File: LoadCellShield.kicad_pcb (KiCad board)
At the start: 2 copper layers, 68.6 x 53.3 mm, 34 parts, among them IC1 INA125, IC2 INA125, J1 Screw_Terminal_01x04, J2 Screw_Terminal_01x04, J7 Barrel_Jack_Switch, P1 Power, P2 Analog, P3 Digital, P4 Digital, P5 CONN_01X01, P6 CONN_01X01, P7 CONN_01X01, P8 CONN_01X01, U1 R-78E5.0-0.5

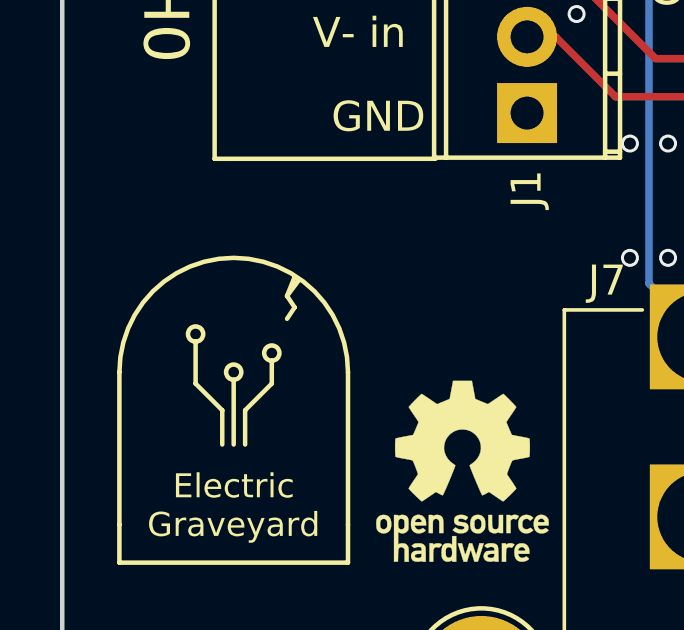
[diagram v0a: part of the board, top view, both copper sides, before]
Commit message: Initial Commit
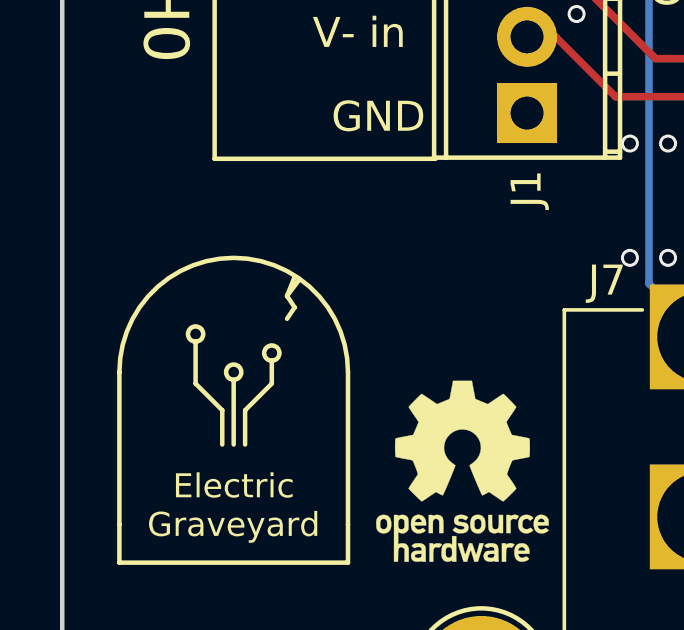
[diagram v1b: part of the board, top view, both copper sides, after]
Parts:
- C1, C2: value C -> 0.1uF
- C3: value C -> 1.0uF
- IC1, IC2: value INA125 -> INA125 (INA125UA/2K5)
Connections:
- J7 pad 3: Net-(J7-Pad3) -> unconnected-(J7-Pad3)
- RV1 pad 1: Net-(RV1-Pad1) -> unconnected-(RV1-Pad1)
- RV2 pad 1: Net-(RV2-Pad1) -> unconnected-(RV2-Pad1)
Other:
- net class Default removed
